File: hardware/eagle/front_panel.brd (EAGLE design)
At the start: 98 x 34 mm, 22 parts, among them IC1 74HCT595N, IC2 74HCT595N

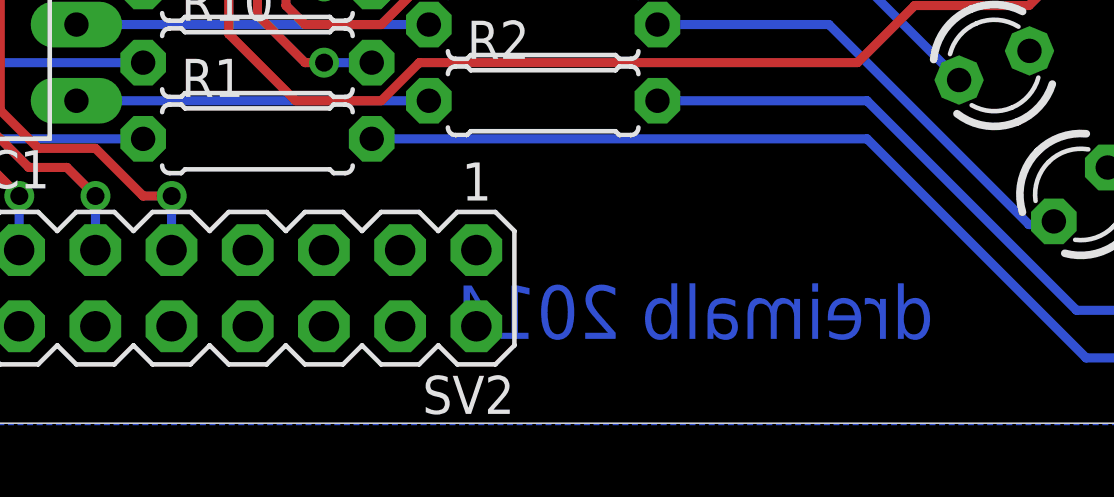
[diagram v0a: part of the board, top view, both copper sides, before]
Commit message: Reorganized project structure.
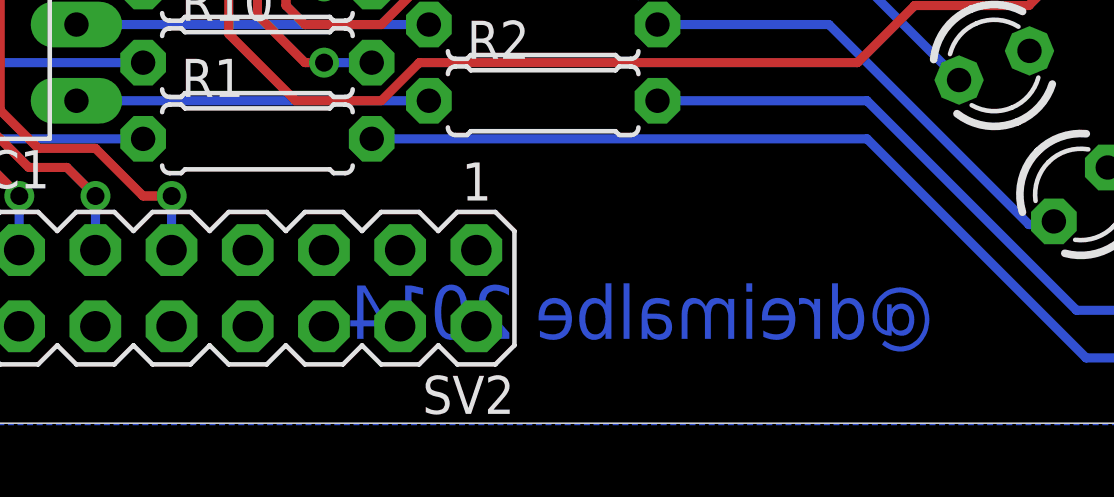
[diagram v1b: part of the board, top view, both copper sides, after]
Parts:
- U$2: device dreimalb:POTI_LED_RING16 -> dreimalbe:POTI_LED_RING16
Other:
- board text added: "@dreimalbe 2014"
- board text removed: "dreimalb 2014"
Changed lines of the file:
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@@
 <wire x1="80.9625" y1="34.0475" x2="97.9625" y2="17.0475" width="0" layer="20" curve="-90"/>
 <wire x1="97.9625" y1="17.0475" x2="80.9625" y2="0.0475" width="0" layer="20" curve="-90"/>
-<text x="66.675" y="2.8575" size="1.778" layer="16" font="vector" ratio="12" rot="MR0">dreimalb 2014</text>
+<text x="66.675" y="2.8575" size="1.778" layer="16" font="vector" ratio="12" rot="MR0">@dreimalbe 2014</text>
 </plain>
 <attributes>
@@
 </element>
 <element name="R17" library="resistor" package="0207/7" value="100" x="11.43" y="6.0325" rot="R180"/>
-<element name="U$2" library="dreimalb" package="POTI_LED_RING16" value="LED_RING_16" x="80.9625" y="17.0475"/>
+<element name="U$2" library="dreimalbe" package="POTI_LED_RING16" value="LED_RING_16" x="80.9625" y="17.0475"/>
 <element name="U$3" library="tsop-1" package="TSOP17XX" value="TSOP1738" x="8.89" y="13.335"/>
 </elements>
@@
 <contactref element="U$2" pad="K15"/>
 <contactref element="U$3" pad="GND"/>
-<wire x1="48.89" y1="3.2775" x2="51.43" y2="3.2775" width="0" layer="19" extent="1-1"/>
 <wire x1="46.35" y1="3.2775" x2="48.89" y2="3.2775" width="0" layer="19" extent="1-1"/>
+<wire x1="51.43" y1="3.2775" x2="48.89" y2="3.2775" width="0" layer="19" extent="1-1"/>
 </signal>
 <signal name="N$3">
